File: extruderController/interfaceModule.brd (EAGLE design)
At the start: 72.1 x 17.8 mm, 4 parts, among them IC2 MAX3467CPA, J1 RJ45, J2 USB_B_PTH

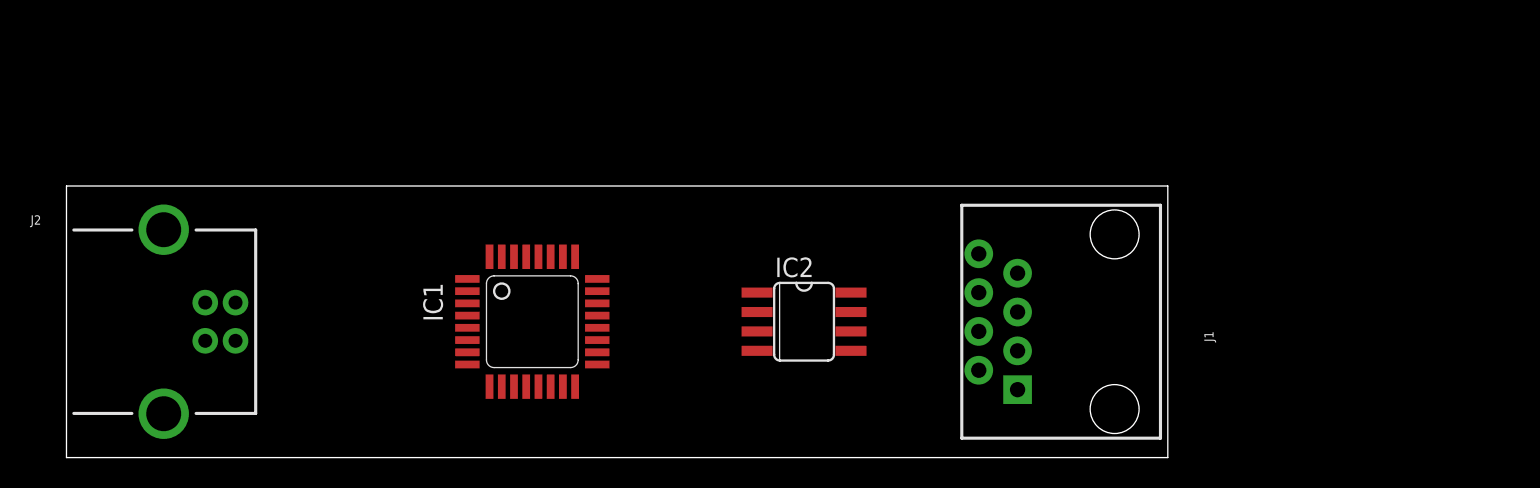
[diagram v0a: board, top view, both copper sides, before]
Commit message: d
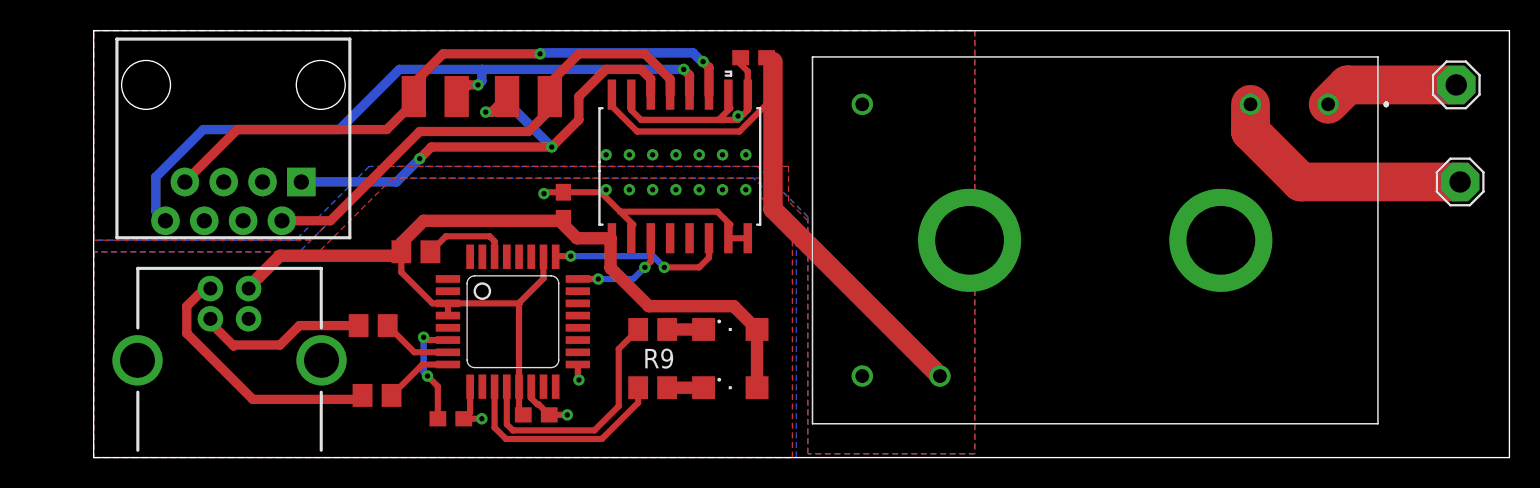
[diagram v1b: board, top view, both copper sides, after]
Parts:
- removed IC2: MAX3467CPA, maxim:SO08
- added C1, C2, C4: 0.1uF, rcl:C0603
- added C3: 33nF, rcl:C0603
- added IC3: ISO3086DW, SamacSys_Parts:SOIC127P1030X265-16N
- added LED1, LED2: (no value), led:SML1206
- added LSP1, LSP2: SE14, solpad:SE14
- added PS1: IRM-03-5, SamacSys_Parts:IRM0312
- added R1, R2: 120, rcl:R1210
- added R5: 470, rcl:R0805
- added R6, R7: 27, rcl:R0805
- added R8, R9: 220, rcl:R0805
- moved J1 59.7 mm to (10.9, 24.4), turned to 180 degrees
- moved J2 6.76 mm to (10.7, 5.08), turned to 90 degrees
- moved IC1 1.27 mm to (29.2, 8.89)
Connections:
- removed net VCC: IC2.1
- removed net VCC1: IC1.3
- removed net VCC2: IC1.26
- new net AGND: C1.2, IC3.10, IC3.15, IC3.9, J1.3, J1.4, J1.5, J1.6, PS1.4
- new net N$1: LSP1.MP, PS1.1
- new net N$10: LED1.C, R8.2
- new net N$2: LSP2.MP, PS1.2
- new net N$3: IC1.8, R6.2
- new net N$4: IC1.30, R5.1
- new net N$5: IC1.7, R7.2
- new net N$6: C3.2, IC1.6
- new net N$7: IC1.12, R8.1
- new net N$8: IC1.11, R9.1
- new net N$9: LED2.C, R9.2
- new net VCC/2: C1.1, IC3.16, PS1.5
- net +5V: now also C2.1, C4.1, IC1.13, IC1.26, IC1.3, IC1.4, IC3.1, LED1.A, LED2.A, R5.2
- net DA: now also IC3.14, R1.2; no longer IC2.8
- net DB: now also IC3.13, R1.1; no longer IC2.7
- net DY: now also IC3.11, R2.1; no longer IC2.5
- net DZ: now also IC3.12, R2.2; no longer IC2.6
- net GND: now also C2.2, C3.1, C4.2, IC1.14, IC1.17, IC1.9, IC3.2, IC3.7, IC3.8; no longer IC2.4
- net RXD: now also IC3.3; no longer IC2.2
- net TXD: now also IC3.6; no longer IC2.3
- net USBD+: now also R7.1
- net USBD-: now also R6.1
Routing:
- net +5V: track 0.00 -> 65.6 mm
- net DZ: track 0.00 -> 45.2 mm, vias 0 -> 2
- net VCC/2: track 0.00 -> 41.0 mm
- net DY: track 0.00 -> 40.7 mm, vias 0 -> 2
- net DA: track 0.00 -> 35.2 mm, vias 0 -> 3
- net DB: track 0.00 -> 32.7 mm
- net GND: track 0.00 -> 25.6 mm, vias 0 -> 11
- net USBD-: track 0.00 -> 17.2 mm
- net N$2: track 0.00 -> 16.9 mm
- net N$7: track 0.00 -> 16.2 mm
- net AGND: track 0.00 -> 14.8 mm, vias 0 -> 8
- net N$8: track 0.00 -> 14.3 mm
- net TXD: track 0.00 -> 11.9 mm, vias 0 -> 2
- net USBD+: track 0.00 -> 11.2 mm
- net N$1: track 0.00 -> 8.91 mm
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- added copper zone on layer 1, net AGND
- added copper zone on layer 16, net AGND
- added copper zone on layer 1, net GND
- added copper zone on layer 16, net GND
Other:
- board size 72.1 x 17.8 mm -> 92.6 x 27.9 mm
